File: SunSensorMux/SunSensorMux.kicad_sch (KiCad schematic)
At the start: 8 parts, among them J1 Conn_01x03, J2 Conn_01x03, U1 TCA9548A_Multiplexer

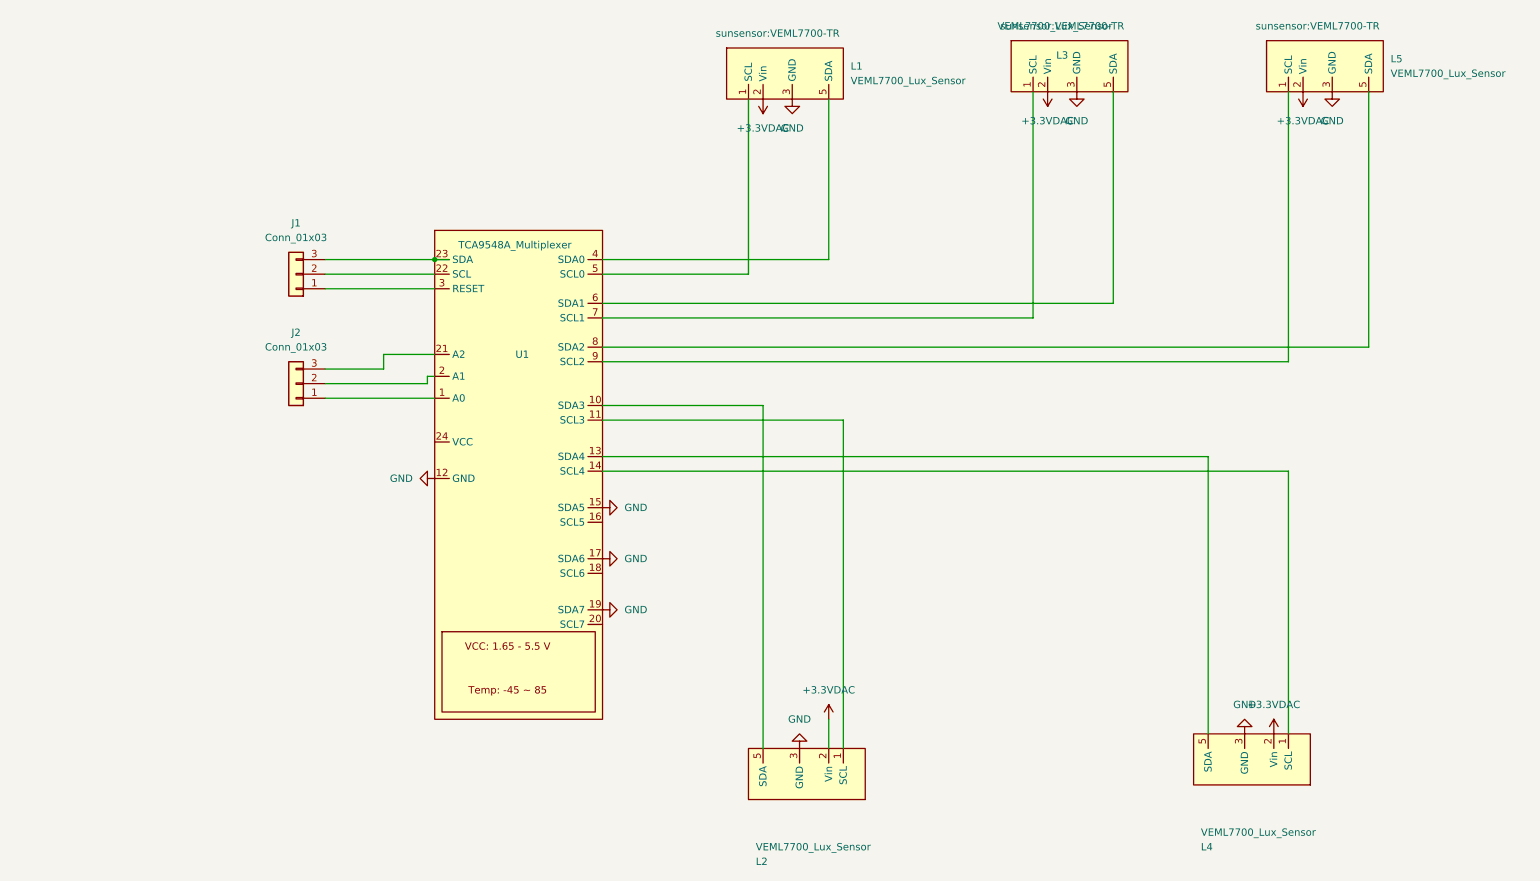
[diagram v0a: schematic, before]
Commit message: finished board
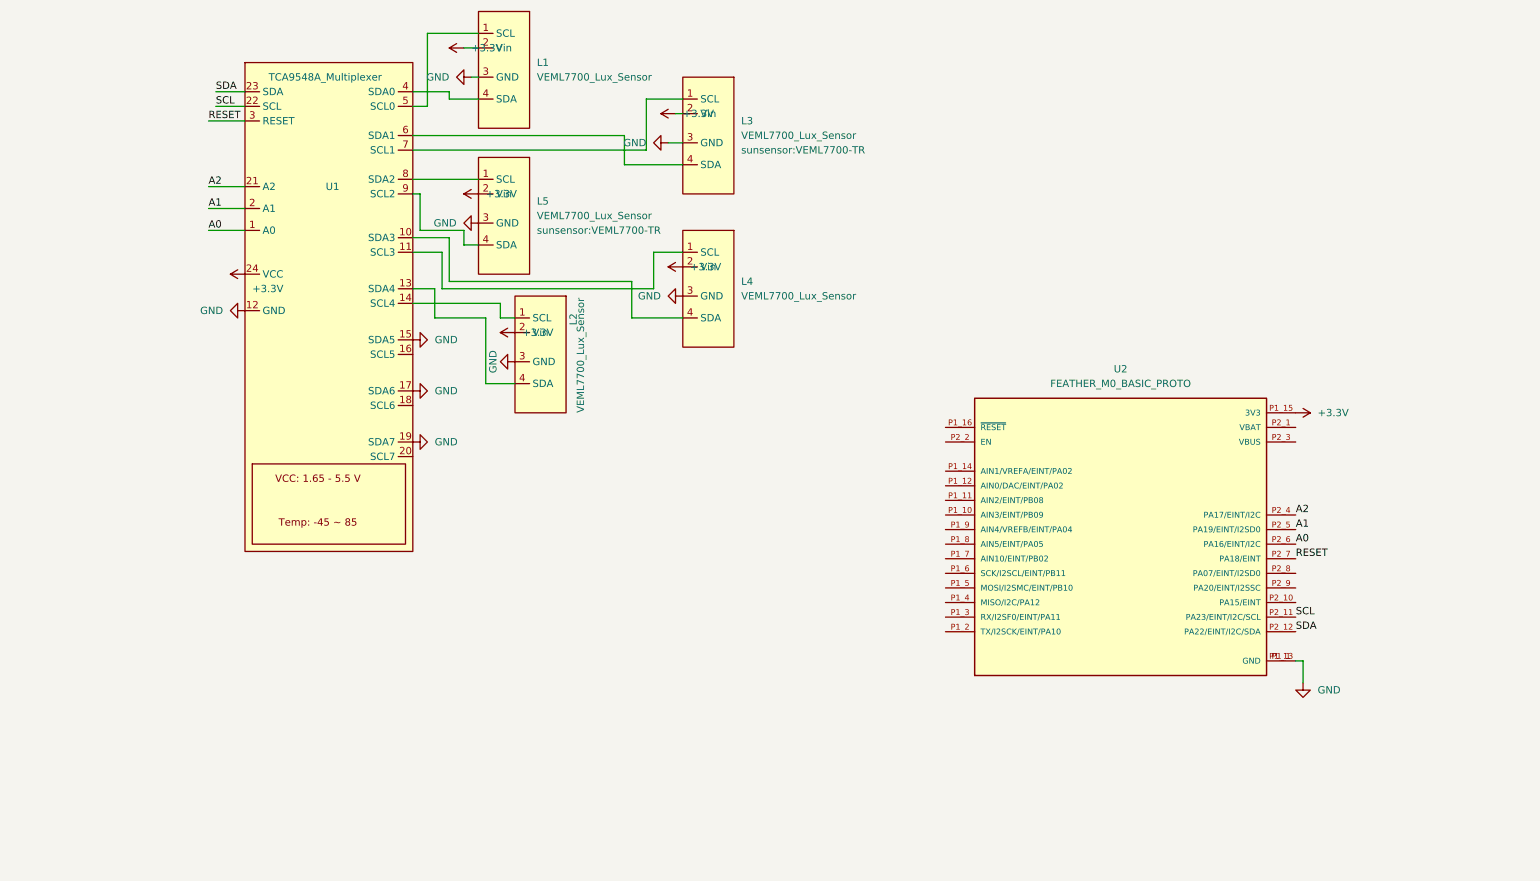
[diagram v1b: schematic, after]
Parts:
- removed J1, J2: Conn_01x03, symbol Connector_Generic:Conn_01x03
- added U2: FEATHER_M0_BASIC_PROTO, sunsensor:MODULE_FEATHER_M0_BASIC_PROTO, symbol sunsensor:FEATHER_M0_BASIC_PROTO
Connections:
- net +3.3VDAC is gone; now on net +3V3: L1.2 (Vin), L2.2 (Vin), L3.2 (Vin), L4.2 (Vin), L5.2 (Vin)
- net GND: now also U2.P1_1 (GND), U2.P1_13 (GND)
- net at L4.1 (SCL): now also U1.11 (SCL3); no longer U1.14 (SCL4)
- net at U1.13 (SDA4): now also L2.4 (SDA); no longer L4.5 (SDA)
- net A0: now reaches U1.1 (A0)
- net A0: now also U2.P2_6 (PA16/EINT/I2C)
- net at U1.10 (SDA3): now also L4.4 (SDA); no longer L2.5 (SDA)
- net at L2.1 (SCL): now also U1.14 (SCL4); no longer U1.11 (SCL3)
- net A1: now reaches U1.2 (A1)
- net A1: now also U2.P2_5 (PA19/EINT/I2SD0)
- net A2: now reaches U1.21 (A2)
- net A2: now also U2.P2_4 (PA17/EINT/I2C)
- net SCL: now reaches U1.22 (SCL)
- net SCL: now also U2.P2_11 (PA23/EINT/I2C/SCL)
- net SDA: now reaches U1.23 (SDA)
- net SDA: now also U2.P2_12 (PA22/EINT/I2C/SDA)
- net +3V3: now reaches U1.24 (VCC)
- net +3V3: now also U2.P1_15 (3V3)
- net RESET: now reaches U1.3 (RESET)
- net RESET: now also U2.P2_7 (PA18/EINT)
- net at U1.4 (SDA0): now also L1.4 (SDA); no longer L1.5 (SDA)
- net at U1.6 (SDA1): now also L3.4 (SDA); no longer L3.5 (SDA)
- net at U1.8 (SDA2): now also L5.1 (SCL); no longer L5.5 (SDA)
- net at U1.9 (SCL2): now also L5.4 (SDA); no longer L5.1 (SCL)
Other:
- moved on the sheet: L1, L3, L4, L5, U1

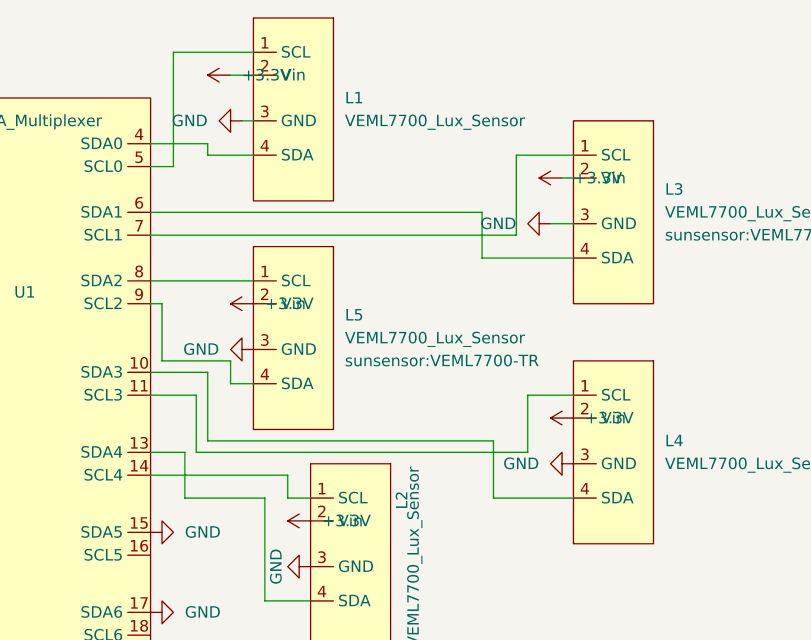
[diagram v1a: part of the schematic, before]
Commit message: Final modifications
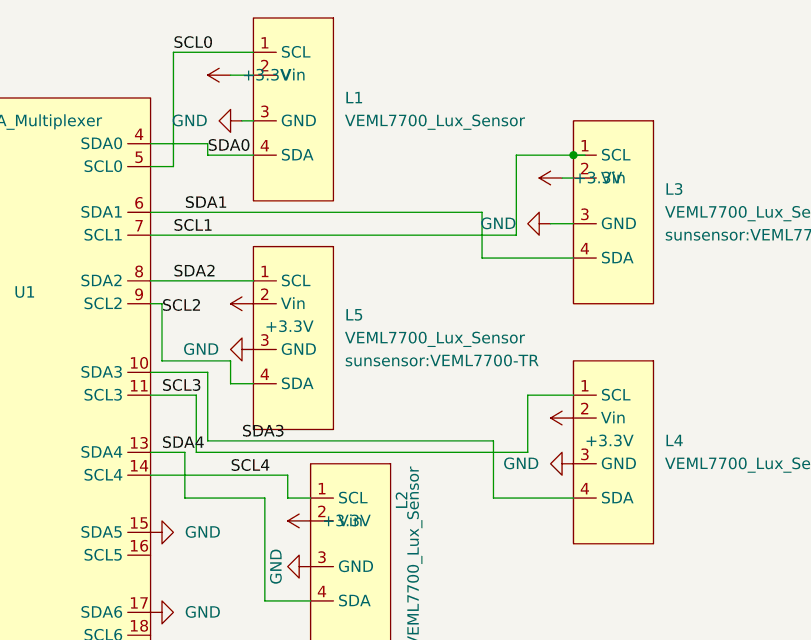
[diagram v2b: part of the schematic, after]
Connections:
- net SCL3: now reaches L4.1 (SCL), U1.11 (SCL3)
- net SDA3: now reaches L4.4 (SDA), U1.10 (SDA3)
- net SDA4: now reaches L2.4 (SDA), U1.13 (SDA4)
- net SCL4: now reaches L2.1 (SCL), U1.14 (SCL4)
- net SDA0: now reaches L1.4 (SDA), U1.4 (SDA0)
- net SCL0: now reaches L1.1 (SCL), U1.5 (SCL0)
- net SDA1: now reaches L3.4 (SDA), U1.6 (SDA1)
- net SCL1: now reaches L3.1 (SCL), U1.7 (SCL1)
- net SDA2: now reaches L5.1 (SCL), U1.8 (SDA2)
- net SCL2: now reaches L5.4 (SDA), U1.9 (SCL2)
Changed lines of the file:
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@@
 (kicad_sch (version 20211123) (generator eeschema)
   (paper "A4")
+  (junction (at 104.14 30.48) (diameter 0) (color 0 0 0 0)
+  )
   (wire (pts (xy 57.15 63.5) (xy 60.96 63.5))
     (stroke (width 0) (type default) (color 0 0 0 0))
@@
     (stroke (width 0) (type default) (color 0 0 0 0))
   )
+  (wire (pts (xy 105.41 30.48) (xy 104.14 30.48))
+    (stroke (width 0) (type default) (color 0 0 0 0))
+  )
   (wire (pts (xy 93.98 41.91) (xy 104.14 41.91))
     (stroke (width 0) (type default) (color 0 0 0 0))
@@
     (effects (font (size 1.27 1.27)) (justify left bottom))
   )
+  (label "SDA1" (at 60.96 36.83 0)
+    (effects (font (size 1.27 1.27)) (justify left bottom))
+  )
   (label "A1" (at 21.59 49.53 0)
     (effects (font (size 1.27 1.27)) (justify left bottom))
   )
+  (label "SDA3" (at 67.31 62.23 0)
+    (effects (font (size 1.27 1.27)) (justify left bottom))
+  )
+  (label "SCL3" (at 58.42 57.15 0)
+    (effects (font (size 1.27 1.27)) (justify left bottom))
+  )
+  (label "SCL4" (at 66.04 66.04 0)
+    (effects (font (size 1.27 1.27)) (justify left bottom))
+  )
   (label "A2" (at 21.59 45.72 0)
     (effects (font (size 1.27 1.27)) (justify left bottom))
   )
+  (label "SDA4" (at 58.42 63.5 0)
+    (effects (font (size 1.27 1.27)) (justify left bottom))
+  )
   (label "A0" (at 21.59 53.34 0)
     (effects (font (size 1.27 1.27)) (justify left bottom))
@@
     (effects (font (size 1.27 1.27)) (justify left bottom))
   )
+  (label "SCL0" (at 59.69 19.05 0)
+    (effects (font (size 1.27 1.27)) (justify left bottom))
+  )
   (label "RESET" (at 210.82 110.49 0)
     (effects (font (size 1.27 1.27)) (justify left bottom))
@@
     (effects (font (size 1.27 1.27)) (justify left bottom))
   )
+  (label "SCL1" (at 59.69 39.37 0)
+    (effects (font (size 1.27 1.27)) (justify left bottom))
+  )
   (label "SCL" (at 22.86 31.75 0)
     (effects (font (size 1.27 1.27)) (justify left bottom))
   )
   (label "A0" (at 210.82 107.95 0)
+    (effects (font (size 1.27 1.27)) (justify left bottom))
+  )
+  (label "SDA0" (at 63.5 30.48 0)
+    (effects (font (size 1.27 1.27)) (justify left bottom))
+  )
+  (label "SDA2" (at 59.69 44.45 0)
+    (effects (font (size 1.27 1.27)) (justify left bottom))
+  )
+  (label "SCL2" (at 58.42 48.26 0)
     (effects (font (size 1.27 1.27)) (justify left bottom))
   )
@@
   )
   (symbol (lib_id "power:+3.3V") (at 104.14 59.69 90) (unit 1)
-    (in_bom yes) (on_board yes) (fields_autoplaced)
+    (in_bom yes) (on_board yes)
     (property "Reference" "#PWR0108" (id 0) (at 107.95 59.69 0)
       (effects (font (size 1.27 1.27)) hide)
     )
-    (property "Value" "+3.3V" (id 1) (at 105.41 59.6899 90)
+    (property "Value" "+3.3V" (id 1) (at 105.41 62.23 90)
       (effects (font (size 1.27 1.27)) (justify right))
     )
@@
   )
   (symbol (lib_id "power:+3.3V") (at 68.58 46.99 90) (unit 1)
-    (in_bom yes) (on_board yes) (fields_autoplaced)
+    (in_bom yes) (on_board yes)
     (property "Reference" "#PWR0101" (id 0) (at 72.39 46.99 0)
       (effects (font (size 1.27 1.27)) hide)
     )
-    (property "Value" "+3.3V" (id 1) (at 69.85 46.9899 90)
-      (effects (font (size 1.27 1.27)) (justify right))
-    )
+    (property "Value" "+3.3V" (id 1) (at 69.85 49.53 90)
+      (effects (font (size 1.27 1.27)) (justify right))
+    )
